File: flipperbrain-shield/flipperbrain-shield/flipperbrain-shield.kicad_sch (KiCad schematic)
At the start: 24 parts, among them J1 Power, J2 Digital/PWM, J3 Analog, J4 Digital/PWM, J5 Screw_Terminal_01x06, J6 Screw_Terminal_01x06, SW10 SW_Push, SW11 SW_Push, SW12 SW_Push, SW13 SW_Push, SW8 SW_Push, SW9 SW_Push

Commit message: nc
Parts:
- J5, J6: footprint TerminalBlock_Phoenix:TerminalBlock_Phoenix_MPT-0,5-6-2.54_1x06_P2.54mm_Horizontal -> TerminalBlock_Phoenix:TerminalBlock_Phoenix_PT-1,5-6-3.5-H_1x06_P3.50mm_Horizontal
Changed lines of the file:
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@@
       (effects (font (size 1.27 1.27)) (justify left))
     )
-    (property "Footprint" "TerminalBlock_Phoenix:TerminalBlock_Phoenix_MPT-0,5-6-2.54_1x06_P2.54mm_Horizontal" (at 201.93 134.62 0)
-      (effects (font (size 1.27 1.27)) hide)
-    )
-    (property "Datasheet" "~" (at 201.93 134.62 0)
+    (property "Footprint" "TerminalBlock_Phoenix:TerminalBlock_Phoenix_PT-1,5-6-3.5-H_1x06_P3.50mm_Horizontal" (at 201.93 134.62 0)
+      (effects (font (size 1.27 1.27)) hide)
+    )
+    (property "Datasheet" "" (at 201.93 134.62 0)
       (effects (font (size 1.27 1.27)) hide)
     )
@@
       (effects (font (size 1.27 1.27)) (justify left))
     )
-    (property "Footprint" "TerminalBlock_Phoenix:TerminalBlock_Phoenix_MPT-0,5-6-2.54_1x06_P2.54mm_Horizontal" (at 208.28 58.42 0)
-      (effects (font (size 1.27 1.27)) hide)
-    )
-    (property "Datasheet" "~" (at 208.28 58.42 0)
-      (effects (font (size 1.27 1.27)) hide)
-    )
+    (property "Footprint" "TerminalBlock_Phoenix:TerminalBlock_Phoenix_PT-1,5-6-3.5-H_1x06_P3.50mm_Horizontal" (at 208.28 58.42 0)
+      (effects (font (size 1.27 1.27)) hide)
+    )
+    (property "Datasheet" "" (at 208.28 58.42 0)
+      (effects (font (size 1.27 1.27)) hide)
+    )

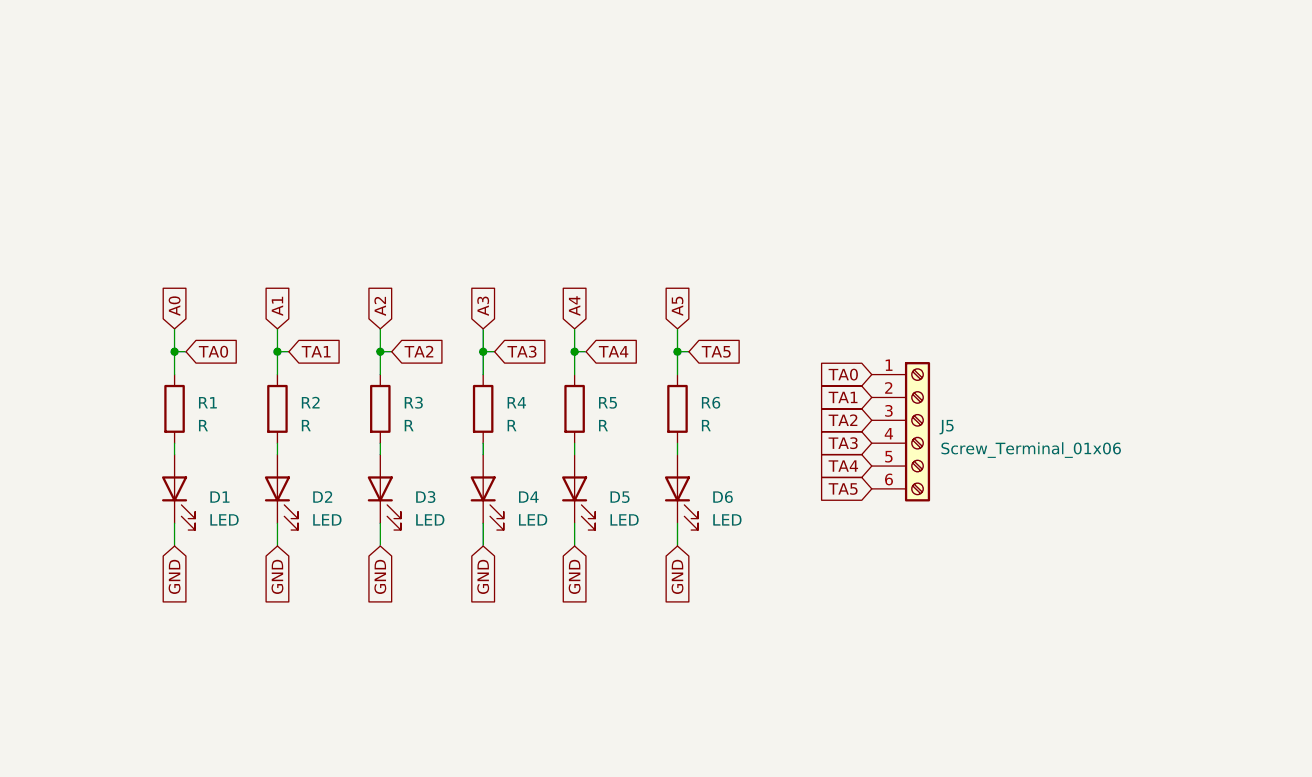
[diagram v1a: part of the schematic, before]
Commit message: nc
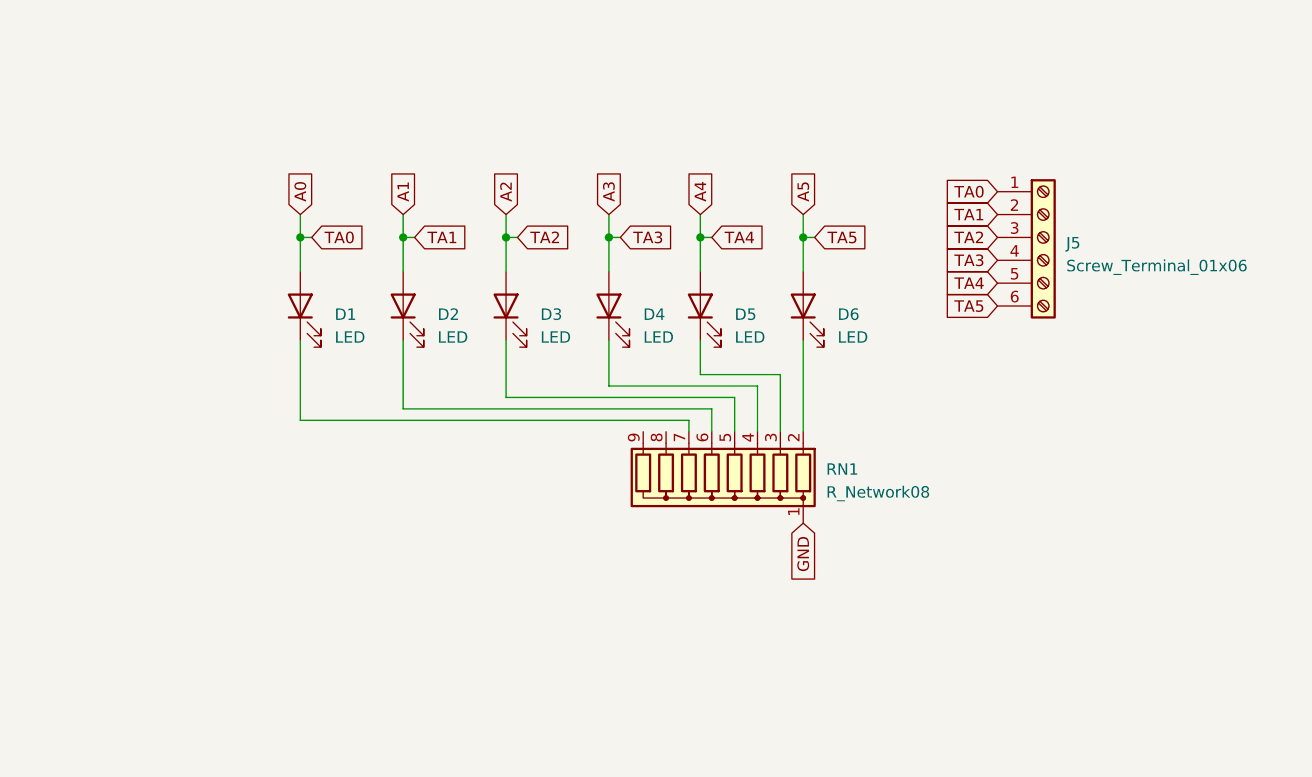
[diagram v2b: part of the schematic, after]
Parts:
- removed R1, R2, R3, R4, R5, R6: R, Resistor_THT:R_Axial_DIN0207_L6.3mm_D2.5mm_P10.16mm_Horizontal, symbol Device:R
- added RN1: R_Network08, Resistor_THT:R_Array_SIP9, symbol Device:R_Network08
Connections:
- net A0: now also D1.2 (A)
- net A1: now also D2.2 (A)
- net A2: now also D3.2 (A)
- net A3: now also D4.2 (A)
- net A4: now also D5.2 (A)
- net A5: now also D6.2 (A)
- net GND: now also RN1.1 (common); no longer D1.1 (K), D2.1 (K), D3.1 (K), D4.1 (K), D5.1 (K), D6.1 (K)
- new net: D5.1 (K), RN1.3 (R2)
- new net: D6.1 (K), RN1.2 (R1)
- new net: D4.1 (K), RN1.4 (R3)
- new net: D3.1 (K), RN1.5 (R4)
- new net: D2.1 (K), RN1.6 (R5)
- new net: D1.1 (K), RN1.7 (R6)
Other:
- moved on the sheet: D1, D2, D3, D4, D5, D6, J5

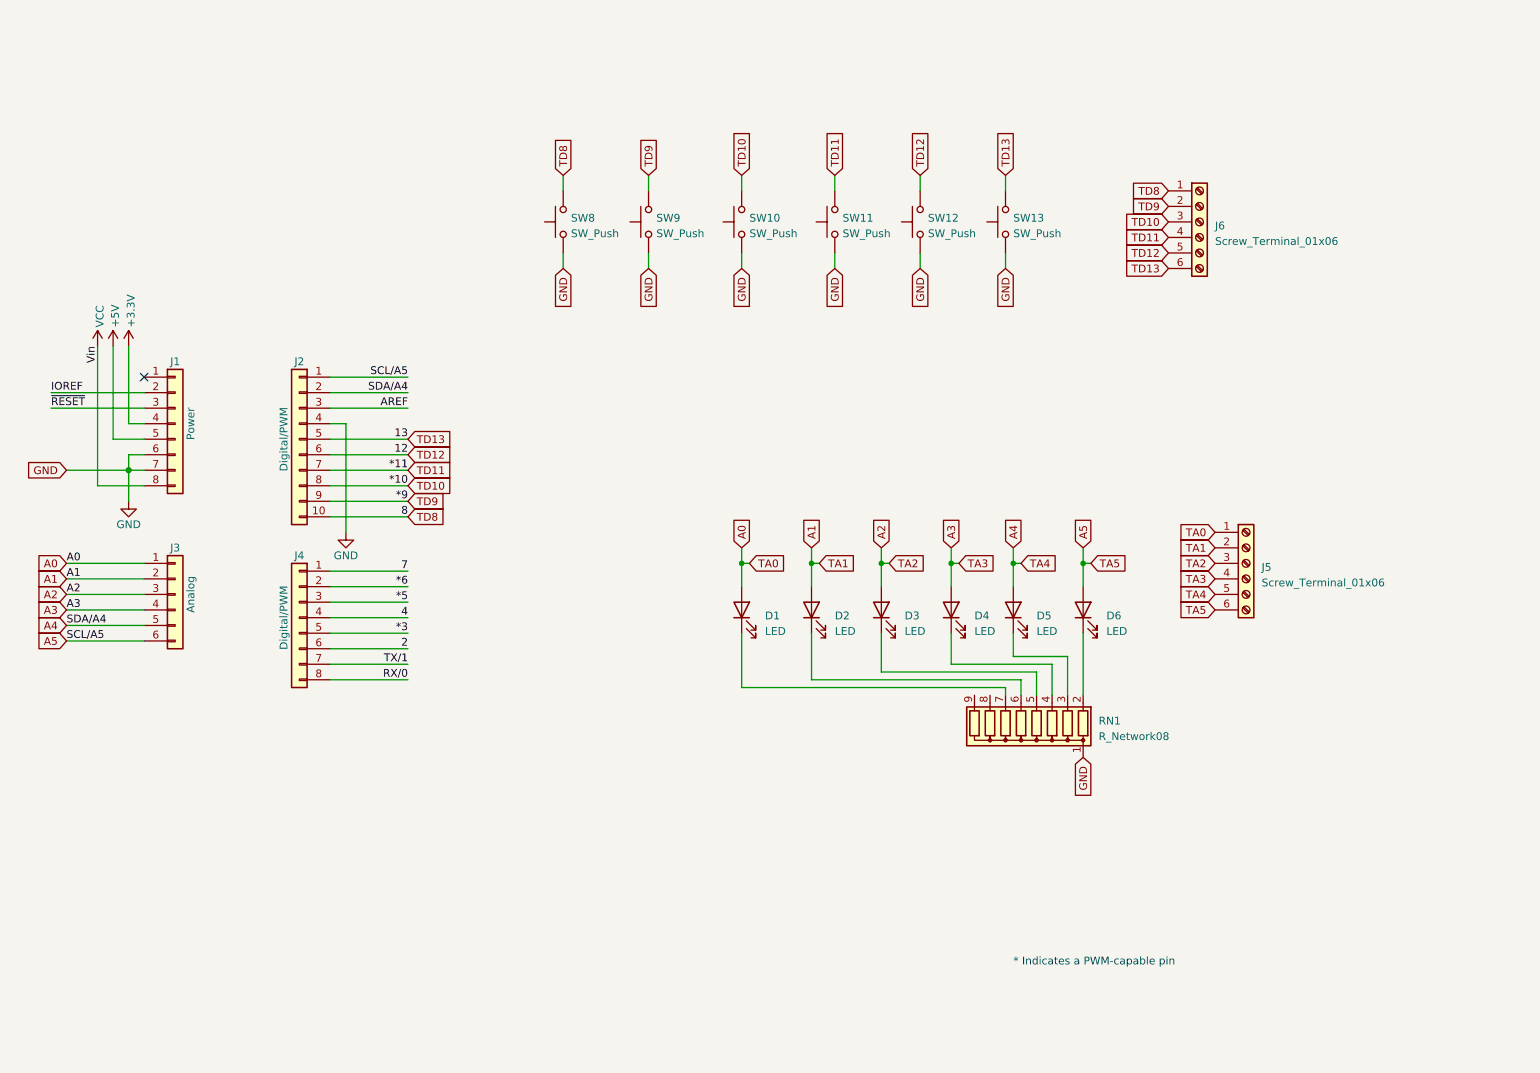
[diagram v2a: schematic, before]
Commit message: nc
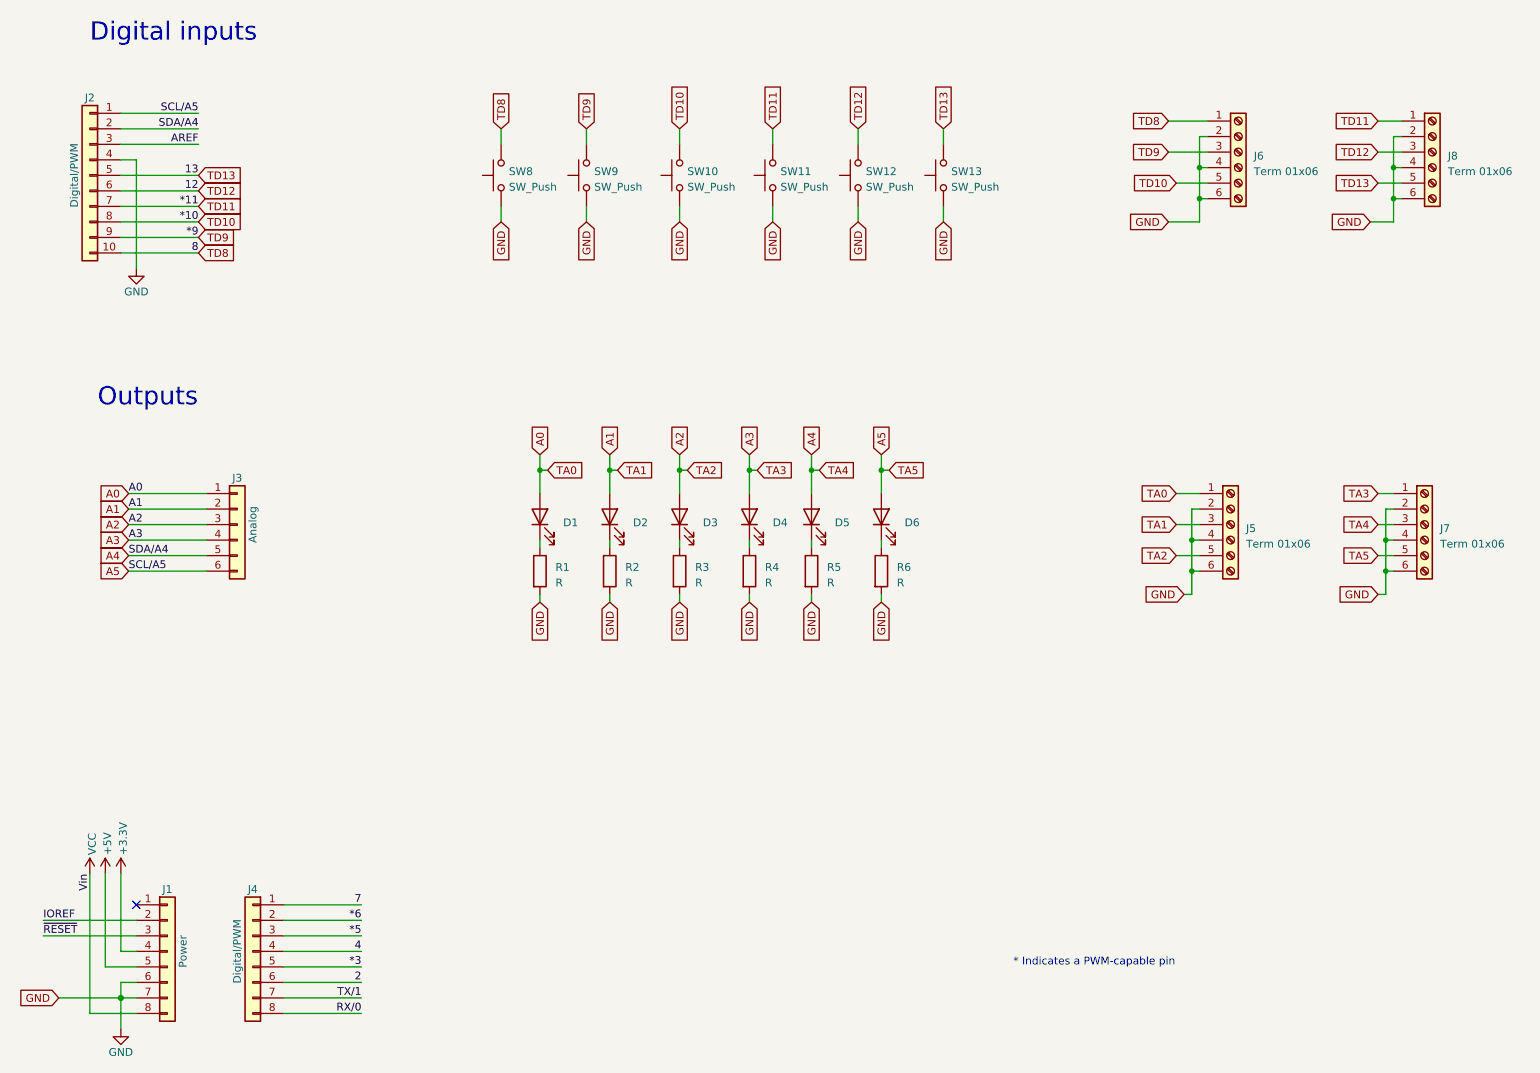
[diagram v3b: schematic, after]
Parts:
- removed RN1: R_Network08, Resistor_THT:R_Array_SIP9, symbol Device:R_Network08
- added J7, J8: Term 01x06, TerminalBlock_Phoenix:TerminalBlock_Phoenix_PT-1,5-6-3.5-H_1x06_P3.50mm_Horizontal, symbol Connector:Screw_Terminal_01x06
- added R1, R2, R3, R4, R5, R6: R, Resistor_THT:R_Axial_DIN0207_L6.3mm_D2.5mm_P7.62mm_Horizontal, symbol Device:R
- J5, J6: value Screw_Terminal_01x06 -> Term 01x06
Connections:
- net A1: now also J5.3 (Pin_3); no longer J5.2 (Pin_2)
- net A2: now also J5.5 (Pin_5); no longer J5.3 (Pin_3)
- net A3: now also J7.1 (Pin_1); no longer J5.4 (Pin_4)
- net A4: now also J7.3 (Pin_3); no longer J5.5 (Pin_5)
- net A5: now also J7.5 (Pin_5); no longer J5.6 (Pin_6)
- net GND: now also J5.2 (Pin_2), J5.4 (Pin_4), J5.6 (Pin_6), J6.2 (Pin_2), J6.4 (Pin_4), J6.6 (Pin_6), J7.2 (Pin_2), J7.4 (Pin_4), J7.6 (Pin_6), J8.2 (Pin_2), J8.4 (Pin_4), J8.6 (Pin_6), R1.2, R2.2, R3.2, R4.2, R5.2, R6.2
- net TD10: now also J6.5 (Pin_5); no longer J6.3 (Pin_3)
- net TD11: now also J8.1 (Pin_1); no longer J6.4 (Pin_4)
- net TD12: now also J8.3 (Pin_3); no longer J6.5 (Pin_5)
- net TD13: now also J8.5 (Pin_5); no longer J6.6 (Pin_6)
- net TD9: now also J6.3 (Pin_3); no longer J6.2 (Pin_2)
- net at D5.1 (K): now also R5.1
- net at D6.1 (K): now also R6.1
- net at D4.1 (K): now also R4.1
- net at D3.1 (K): now also R3.1
- net at D2.1 (K): now also R2.1
- net at D1.1 (K): now also R1.1
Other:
- note added: "Digital inputs"
- note added: "Outputs"
- moved on the sheet: D1, D2, D3, D4, D5, D6, J1, J2, J3, J4, J5, J6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
